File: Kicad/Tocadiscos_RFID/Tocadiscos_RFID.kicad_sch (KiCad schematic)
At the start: 7 parts, among them M1 Stepper_Motor_unipolar_5pin, P1 Conn_02x20, P2 Conn_02x20, U1 DFPlayer_MiniMP3, U2 ULN2003

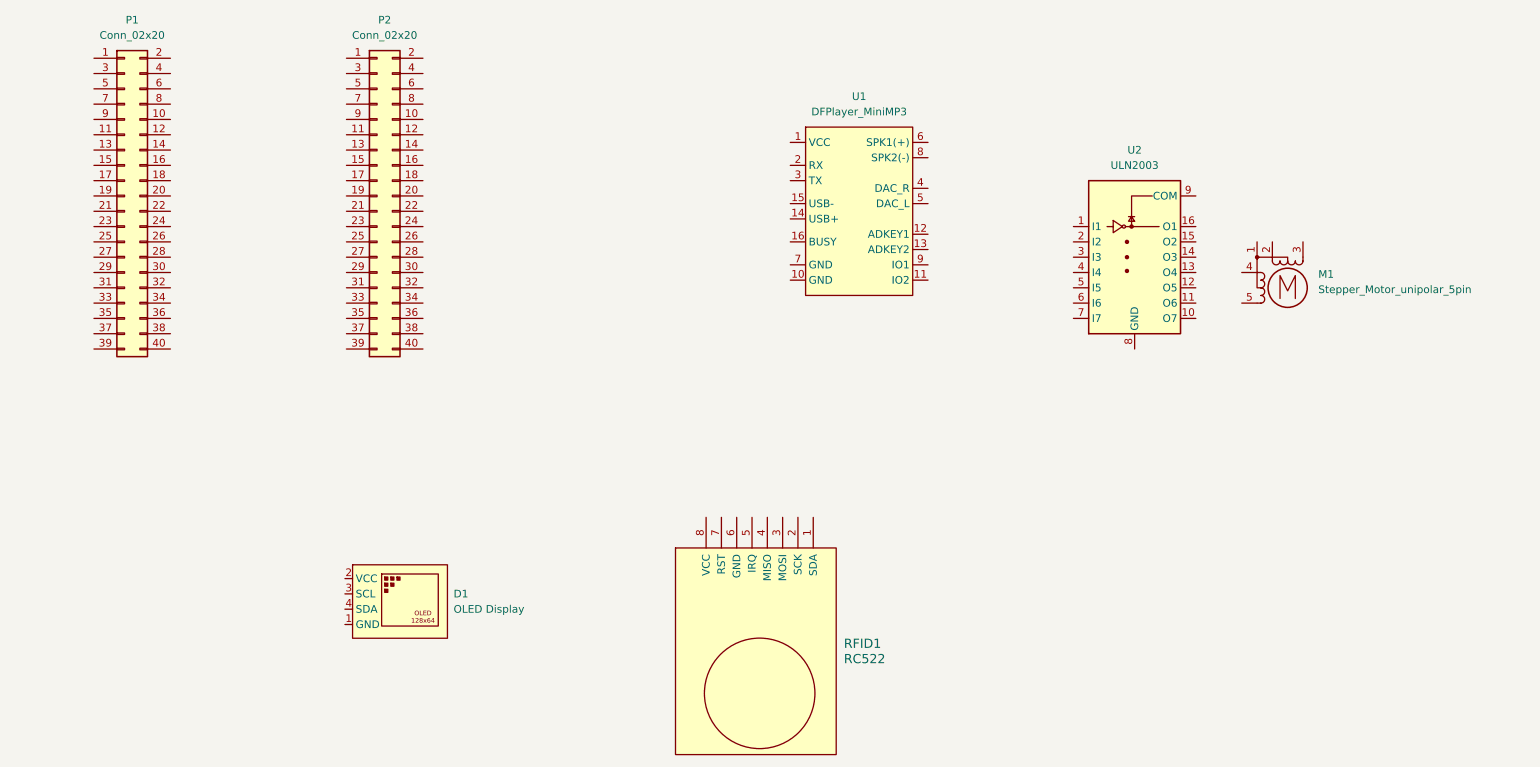
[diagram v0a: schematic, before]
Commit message: pines del motor(que seguro hay que cambiar)
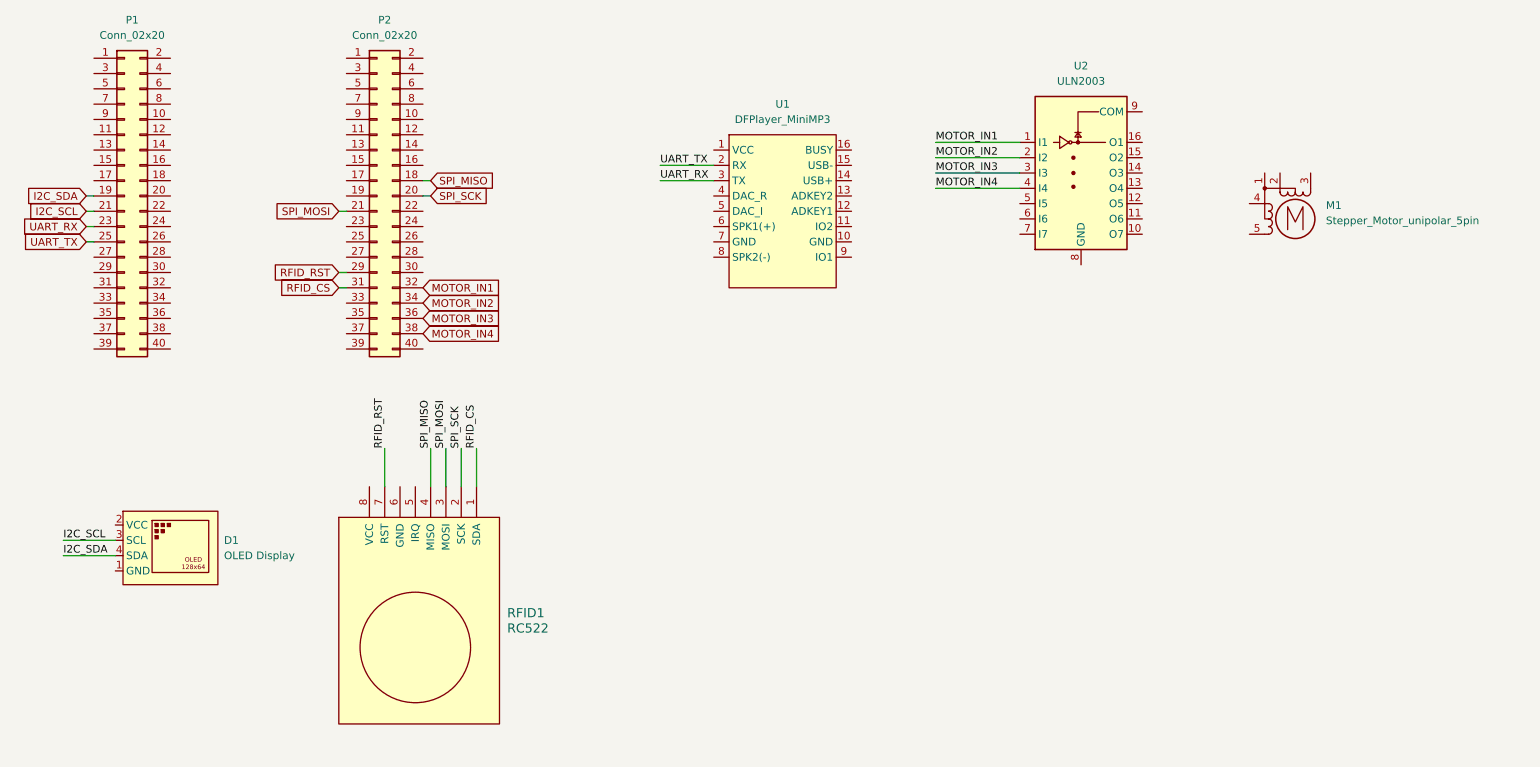
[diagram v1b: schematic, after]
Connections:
- net SPI_MISO: now reaches P2.18 (Pin_18)
- net SPI_MISO: now also RFID1.4 (MISO)
- net SPI_SCK: now reaches P2.20 (Pin_20)
- net SPI_SCK: now also RFID1.2 (SCK)
- net SPI_MOSI: now reaches P2.21 (Pin_21)
- net SPI_MOSI: now also RFID1.3 (MOSI)
- net RFID_RST: now reaches P2.29 (Pin_29)
- net RFID_RST: now also RFID1.7 (RST)
- net RFID_CS: now reaches P2.31 (Pin_31)
- net RFID_CS: now also RFID1.1 (SDA)
- net MOTOR_IN1: now reaches P2.32 (Pin_32)
- net MOTOR_IN1: now also U2.1 (I1)
- net MOTOR_IN2: now reaches P2.34 (Pin_34)
- net MOTOR_IN2: now also U2.2 (I2)
- net MOTOR_IN3: now reaches P2.36 (Pin_36)
- net MOTOR_IN3: now also U2.3 (I3)
- net MOTOR_IN4: now reaches P2.38 (Pin_38)
- net MOTOR_IN4: now also U2.4 (I4)
- net I2C_SCL: now reaches D1.3 (SCL)
- net I2C_SCL: now also P1.21 (Pin_21)
- net I2C_SDA: now reaches D1.4 (SDA)
- net I2C_SDA: now also P1.19 (Pin_19)
- net UART_RX: now reaches P1.23 (Pin_23)
- net UART_RX: now also U1.3 (TX)
- net UART_TX: now reaches P1.25 (Pin_25)
- net UART_TX: now also U1.2 (RX)
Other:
- moved on the sheet: D1, M1, RFID1, U1, U2
